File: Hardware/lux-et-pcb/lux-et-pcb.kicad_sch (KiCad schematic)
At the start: 87 parts, among them J1 Conn_01x03_Socket, J2 Conn_01x03_Socket, J3 Conn_01x03_Socket, J4 USB_C_Receptacle_PowerOnly_6P, Q1 PMOS, Q2 PMOS, Q3 AO3400A, Q4 AO3400A, Q5 AO3400A, Q7 2N7002K, U1 XL1509-5V, U2 AP2112K-3.3, U3 ESP32-WROOM-32, U4 TP4056

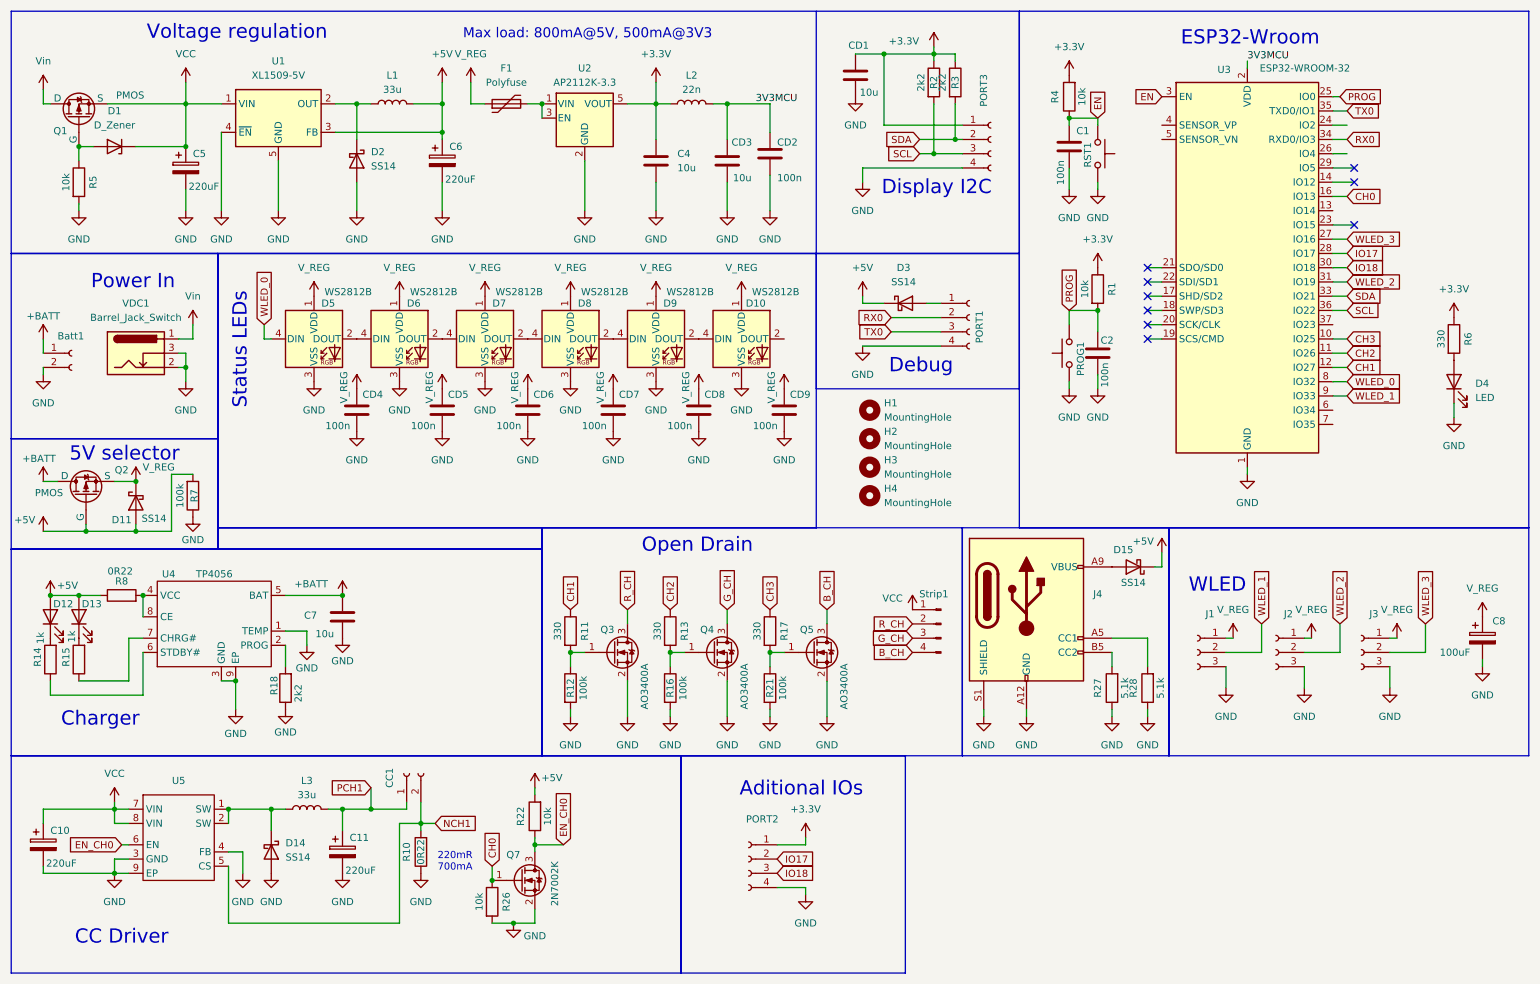
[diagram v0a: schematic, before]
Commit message: BoM update
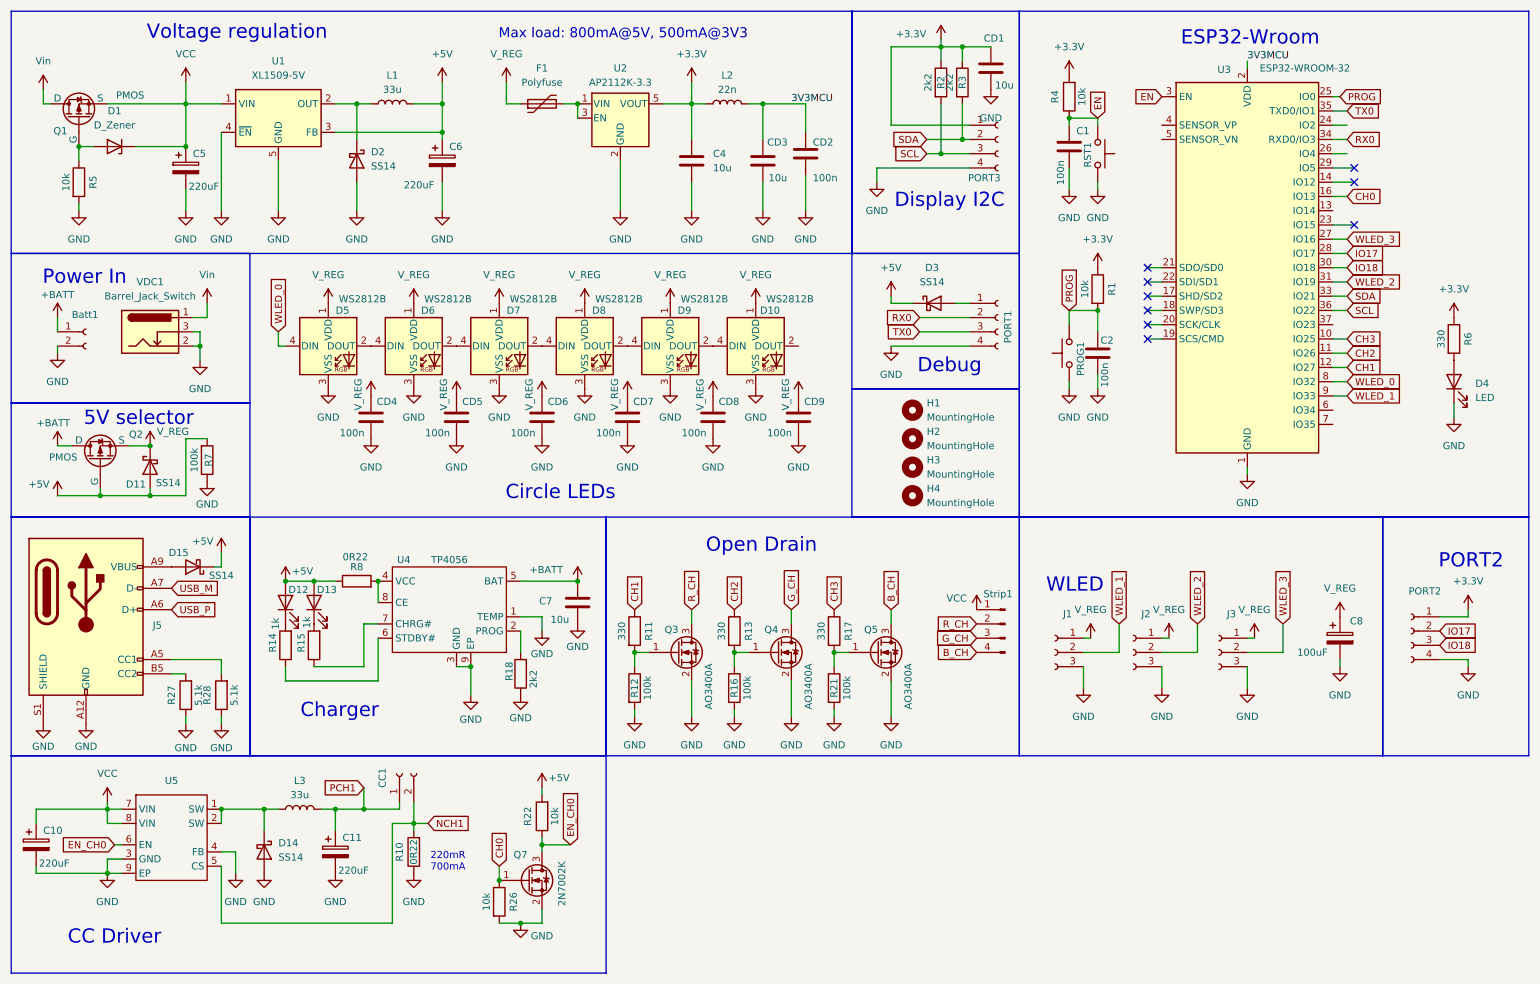
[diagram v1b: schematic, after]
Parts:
- removed J4: USB_C_Receptacle_PowerOnly_6P, Library:USB-C-SMD_GT-USB-7101A, symbol Connector:USB_C_Receptacle_PowerOnly_6P
- added J5: USB_C_Receptacle_USB2.0_8P, Library:USB-C-SMD_GT-USB-7101A, symbol New_Library:USB_C_Receptacle_USB2.0_8P
- C4, CD1, CD3: LCSC C77075 -> C380331
- C7: LCSC C162422 -> C380331
- D10, D5, D6, D7, D8, D9: LCSC 1 -> C2843785
- L2: LCSC 1 -> C108962
- PORT1, PORT3: LCSC 1 -> C7433470
- PORT2: LCSC (none) -> C7433470
- PROG1, RST1: LCSC 1 -> C2888502
- Q3, Q4, Q5: LCSC (none) -> C347497
- R27, R28: LCSC C -> C27834
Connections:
- net GND: now also J5.A12 (GND), J5.B12 (GND), J5.S1 (SHIELD)
- net at R28.2: now also J5.A5 (CC1)
- net at D15.2 (A): now also J5.A9 (VBUS), J5.B9 (VBUS)
- net at R27.2: now also J5.B5 (CC2)
- new net USB_M: J5.A7 (D-)
- new net USB_P: J5.A6 (D+)
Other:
- note added: "Circle LEDs"
- note added: "PORT2"
- note removed: "Aditional IOs"
- note removed: "Status LEDs"
- moved on the sheet: Batt1, C10, C11, C4, C7, C8, CC1, CD1, CD2, CD3, CD4, CD5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
